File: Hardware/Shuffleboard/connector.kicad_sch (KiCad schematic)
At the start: 2 parts, among them J1 1751138, J2 1751138

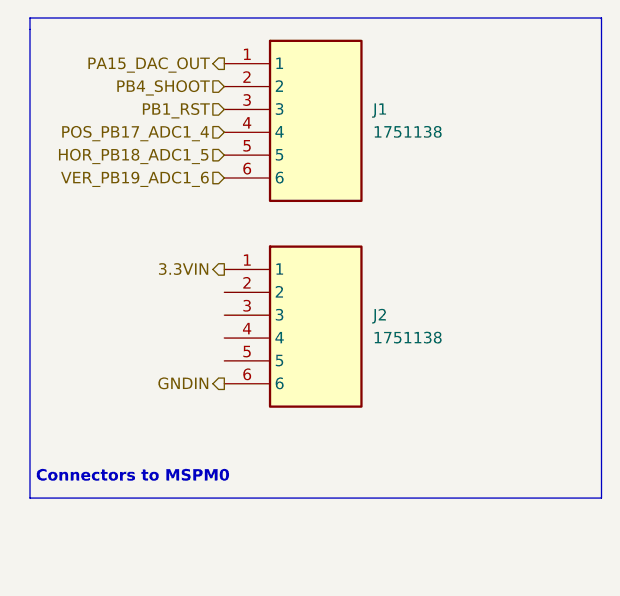
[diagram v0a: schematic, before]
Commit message: led's, mux
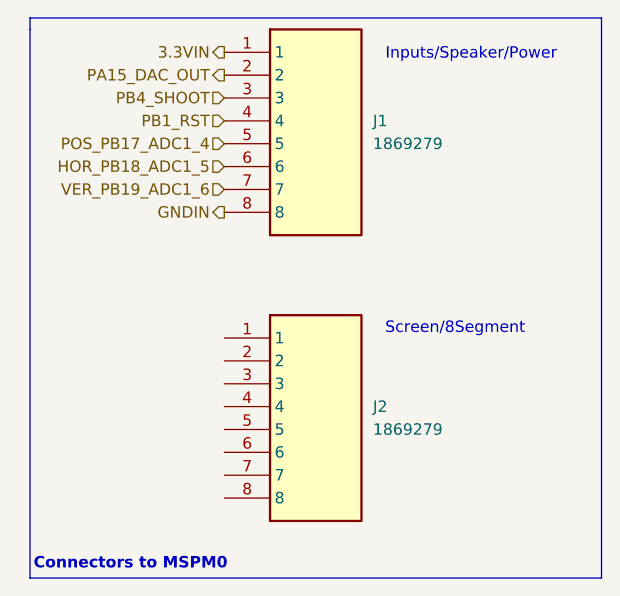
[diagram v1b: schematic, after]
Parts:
- removed J1, J2: 1751138, 1751138, symbol ShuffCon:1751138
- added J1, J2: 1869279, 1869279, symbol ShuffCon:1869279
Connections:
- net 3.3VIN: now also J1.1
- net GNDIN: now also J1.8
- net HOR_PB18_ADC1_5: now also J1.6
- net PA15_DAC_OUT: now also J1.2
- net PB1_RST: now also J1.4
- net PB4_SHOOT: now also J1.3
- net POS_PB17_ADC1_4: now also J1.5
- net VER_PB19_ADC1_6: now also J1.7
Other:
- note added: "Inputs/Speaker/Power"
- note added: "Screen/8Segment"
